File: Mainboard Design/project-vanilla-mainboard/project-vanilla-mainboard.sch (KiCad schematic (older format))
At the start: 60 parts, among them J1 ICSP, J2 USB_B, SW1 OBSF-24, SW10 OBSF-24, SW11 OBSF-24, SW12 OBSF-24, SW13 OBSF-24, SW14 OBSF-24, SW15 OBSF-24, SW16 OBSF-24, SW2 OBSF-24, SW3 OBSF-24, SW4 OBSF-24, SW5 OBSF-24, SW6 OBSF-24, SW7 OBSF-24, SW8 OBSF-24, SW9 OBSF-24, U1 ATmega32U4-AU, U2 TPD3S014, Y1 16Mhz

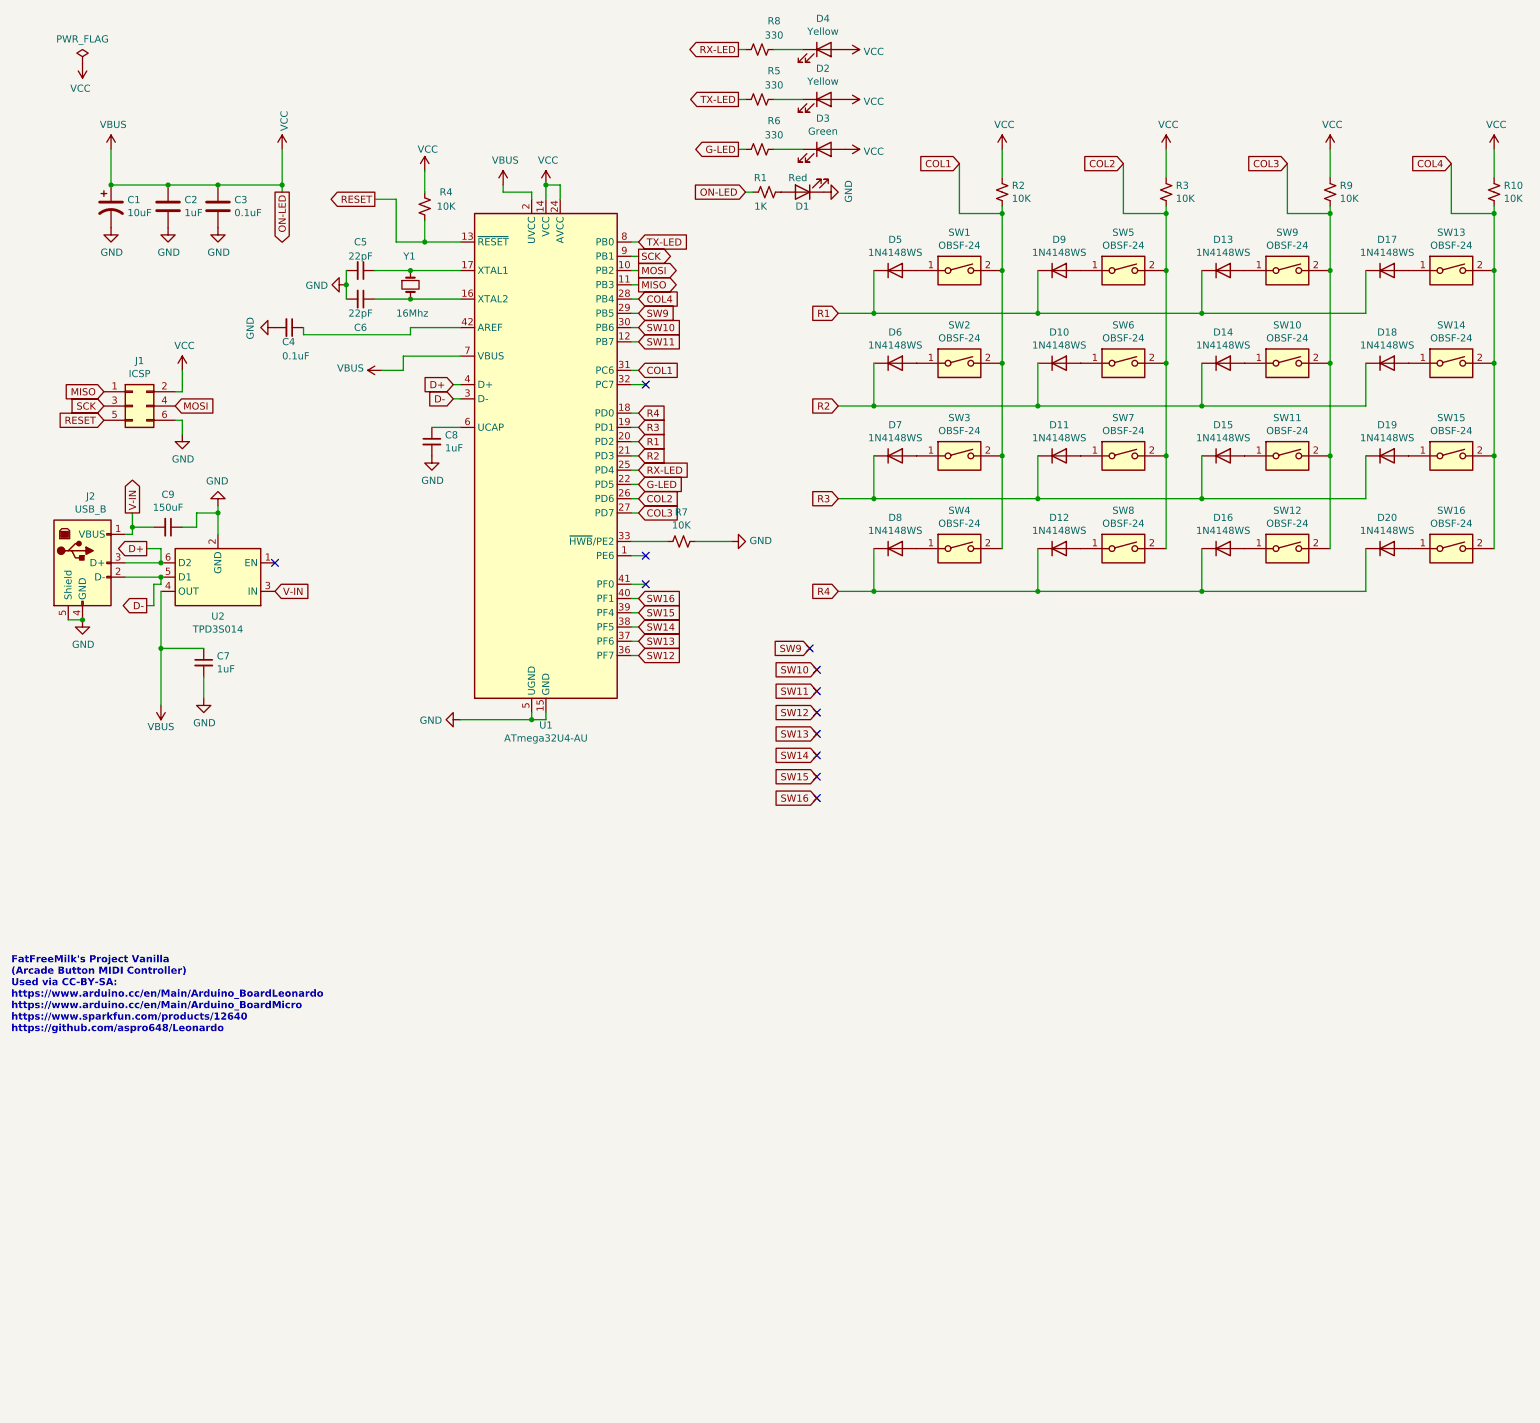
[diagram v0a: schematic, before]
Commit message: A few incrimental updates to the schematic.
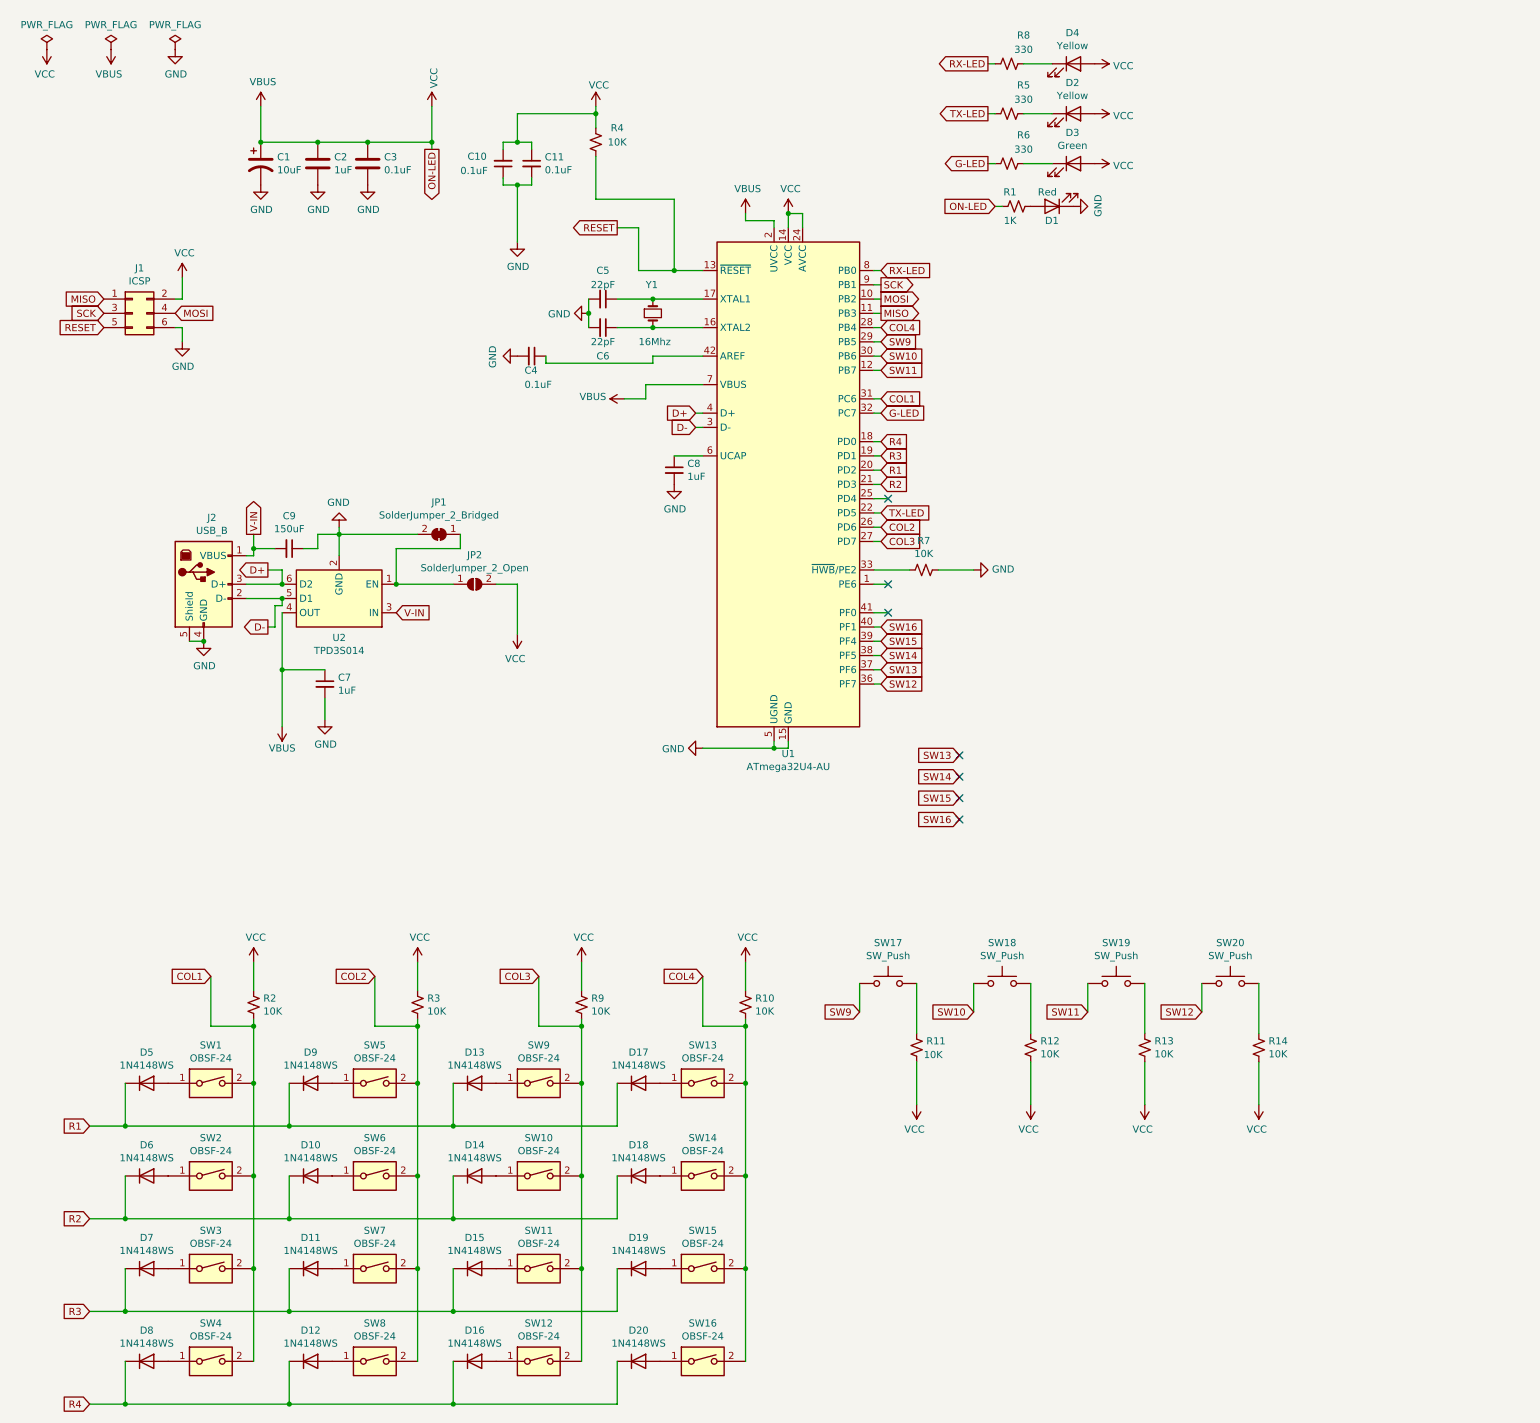
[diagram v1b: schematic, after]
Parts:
- added C10, C11: 0.1uF, symbol Device:C_Small
- added JP1: SolderJumper_2_Bridged, symbol Jumper:SolderJumper_2_Bridged
- added JP2: SolderJumper_2_Open, symbol Jumper:SolderJumper_2_Open
- added R11, R12, R13, R14: 10K, symbol Device:R_Small_US
- added SW17, SW18, SW19, SW20: SW_Push, symbol Switch:SW_Push
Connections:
- net G-LED: now also U1.32 (PC7); no longer U1.22 (PD5)
- net GND: now also C10.1, C11.2, JP1.2 (B)
- net RX-LED: now also U1.8 (PB0); no longer U1.25 (PD4)
- net SW10: now also SW18.1
- net SW11: now also SW19.1
- net SW12: now also SW20.1
- net SW9: now also SW17.1
- net TX-LED: now also U1.22 (PD5); no longer U1.8 (PB0)
- net VBUS: now also C10.2, C11.1, JP2.2 (B), R11.2, R12.1, R13.1, R14.1
- net at U2.1 (EN): now also JP1.1 (A), JP2.1 (A)
- new net: R12.2, SW18.2
- new net: R14.2, SW20.2
- new net: R13.2, SW19.2
- new net: R11.1, SW17.2
- no-connect marks 12 -> 7
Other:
- note removed: "FatFreeMilk's Project Vanilla\n(Arcade Button MIDI Controller)\nUsed via CC-BY-SA:\nhttps://www.arduino.cc/en/Main/Arduino_BoardLeonardo\nhttps://www.arduino.cc/en/Main/Arduino_BoardMicro\nhttps://www.sparkfun.com/products/12640\nhttps://github.com/aspro648/Leonardo"
- moved on the sheet: C1, C2, C3, C4, C5, C6, C7, C8, C9, D1, D2, D3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
